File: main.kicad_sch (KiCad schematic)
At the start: 88 parts, among them J1 USB_C_Receptacle, J2 SPIheader, J3 Bus_PCI_Express_x4, J4 chip-annoyers, J5 UART, J6 I2C, U2 SPI_SOIC-8, U3 SPI_DFN-8, Y1 25MHz

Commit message: component arrangement
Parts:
- R1: footprint Resistor_SMD:R_0201_0603Metric -> Resistor_SMD:R_0402_1005Metric
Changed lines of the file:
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@@
 			)
 		)
-		(property "Footprint" "Resistor_SMD:R_0201_0603Metric"
+		(property "Footprint" "Resistor_SMD:R_0402_1005Metric"
 			(at 378.46 132.08 0)
 			(effects

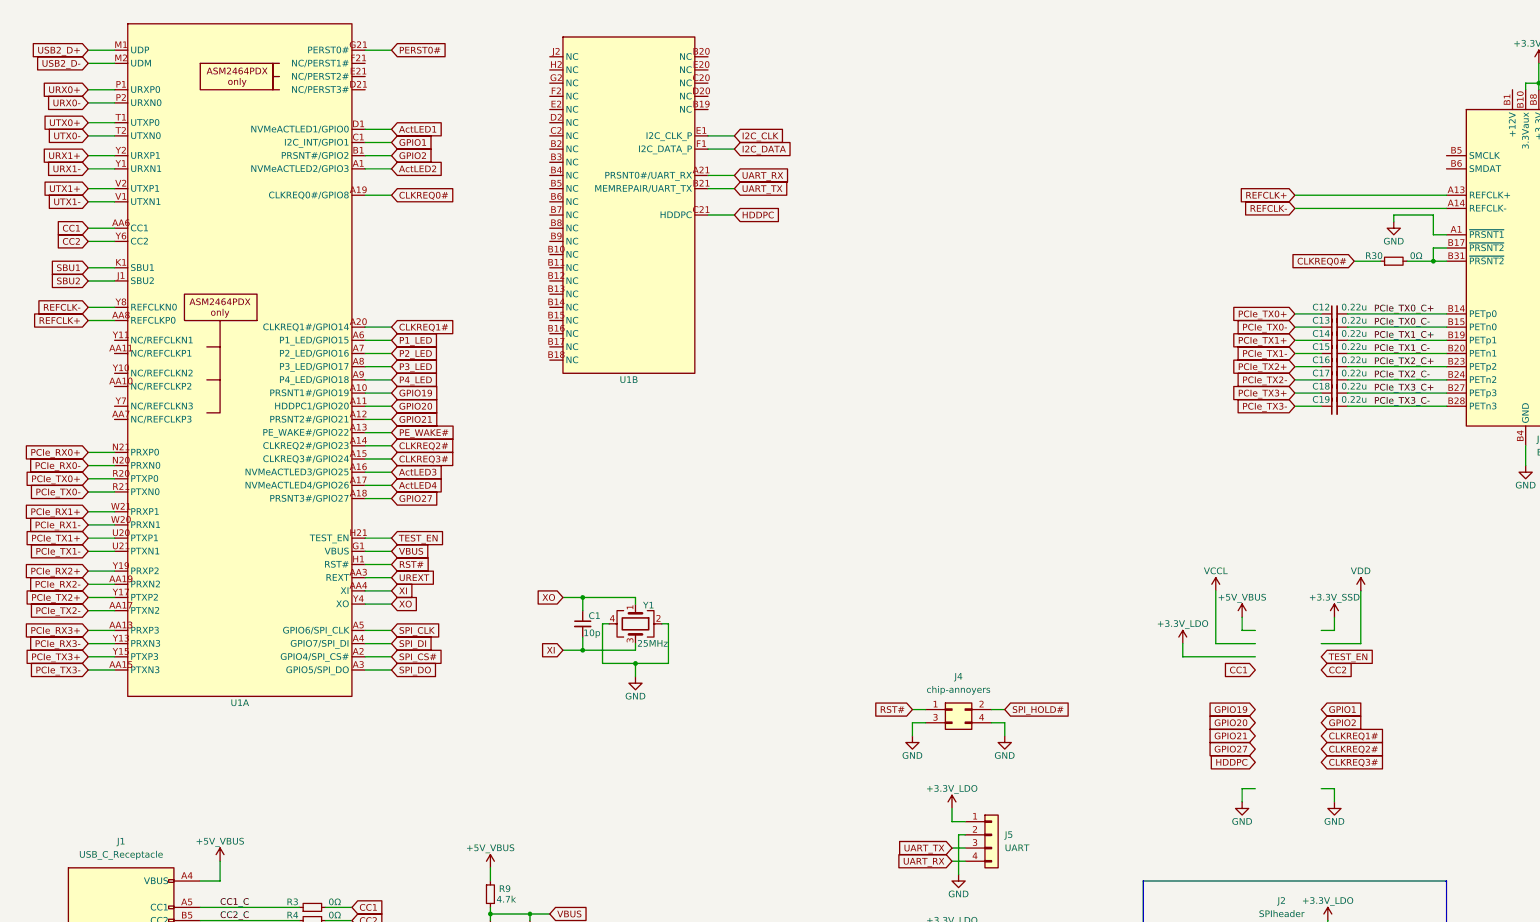
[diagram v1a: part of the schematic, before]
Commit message: A loooot of cool routing and added more connectors
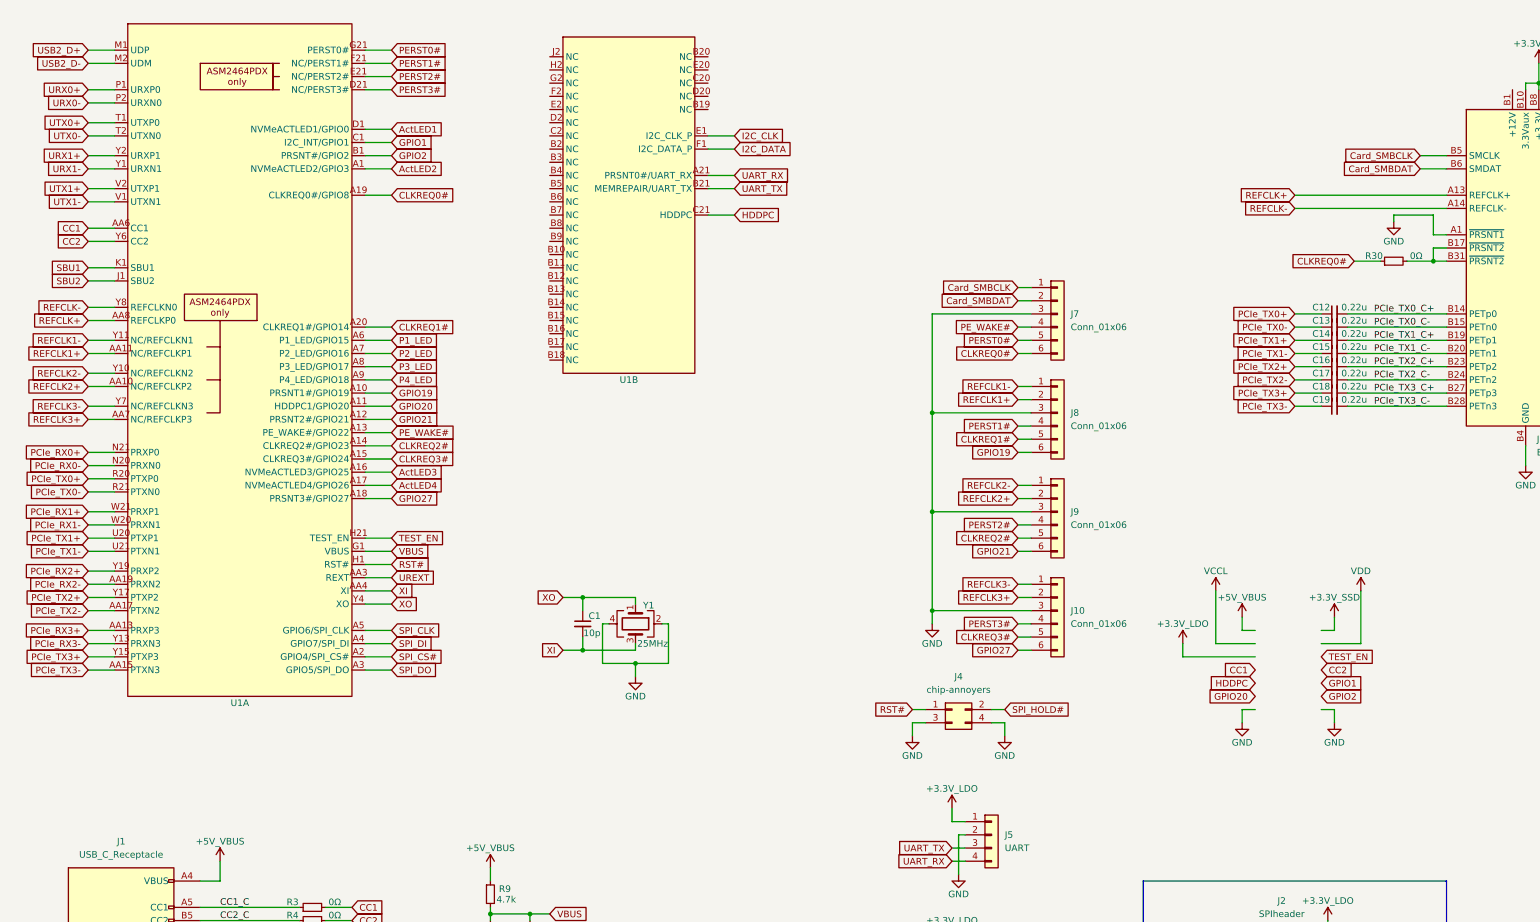
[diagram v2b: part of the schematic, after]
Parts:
- added J10, J7, J8, J9: Conn_01x06, Connector_PinHeader_1.27mm:PinHeader_1x06_P1.27mm_Vertical, symbol Connector_Generic:Conn_01x06
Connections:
- net CLKREQ0#: now also J7.6 (Pin_6)
- net CLKREQ1#: now also J8.5 (Pin_5)
- net CLKREQ2#: now also J9.5 (Pin_5)
- net CLKREQ3#: now also J10.5 (Pin_5)
- net GND: now also J10.3 (Pin_3), J7.3 (Pin_3), J8.3 (Pin_3), J9.3 (Pin_3)
- net GPIO19: now also J8.6 (Pin_6)
- net GPIO21: now also J9.6 (Pin_6)
- net GPIO27: now also J10.6 (Pin_6)
- net PERST0#: now also J7.5 (Pin_5)
- net PE_WAKE#: now also J7.4 (Pin_4)
- net Card_SMBCLK: now reaches J3.B5 (SMCLK)
- net Card_SMBCLK: now also J7.1 (Pin_1)
- net Card_SMBDAT: now reaches J3.B6 (SMDAT)
- net Card_SMBDAT: now also J7.2 (Pin_2)
- net REFCLK2+: now reaches U1.AA10 (NC/REFCLKP2)
- net REFCLK2+: now also J9.2 (Pin_2)
- net REFCLK1+: now reaches U1.AA11 (NC/REFCLKP1)
- net REFCLK1+: now also J8.2 (Pin_2)
- net REFCLK3+: now reaches U1.AA7 (NC/REFCLKP3)
- net REFCLK3+: now also J10.2 (Pin_2)
- net PERST3#: now reaches U1.D21 (NC/PERST3#)
- net PERST3#: now also J10.4 (Pin_4)
- net PERST2#: now reaches U1.E21 (NC/PERST2#)
- net PERST2#: now also J9.4 (Pin_4)
- net PERST1#: now reaches U1.F21 (NC/PERST1#)
- net PERST1#: now also J8.4 (Pin_4)
- net REFCLK2-: now reaches U1.Y10 (NC/REFCLKN2)
- net REFCLK2-: now also J9.1 (Pin_1)
- net REFCLK1-: now reaches U1.Y11 (NC/REFCLKN1)
- net REFCLK1-: now also J8.1 (Pin_1)
- net REFCLK3-: now reaches U1.Y7 (NC/REFCLKN3)
- net REFCLK3-: now also J10.1 (Pin_1)
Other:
- company: (none) -> WifiCable

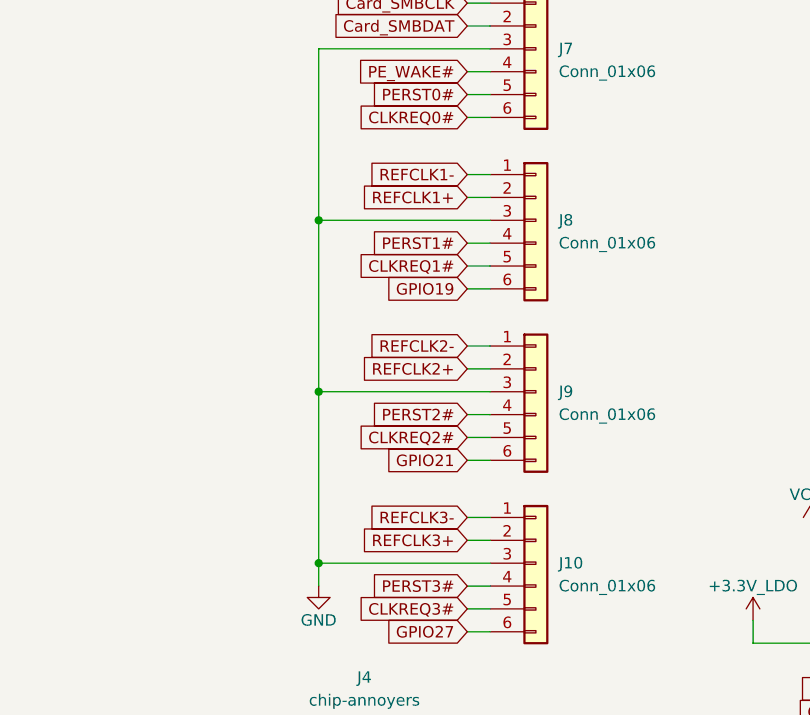
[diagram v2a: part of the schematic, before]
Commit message: Horrible nightmare routing
oh my stars will it do gen 4?
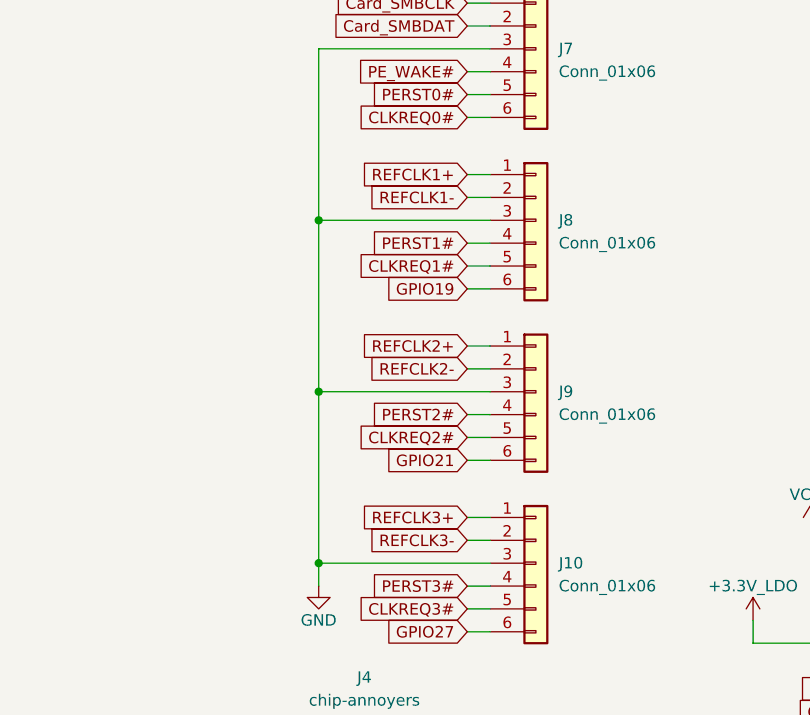
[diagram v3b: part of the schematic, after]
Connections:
- net REFCLK1+: now also J8.1 (Pin_1); no longer J8.2 (Pin_2)
- net REFCLK1-: now also J8.2 (Pin_2); no longer J8.1 (Pin_1)
- net REFCLK2+: now also J9.1 (Pin_1); no longer J9.2 (Pin_2)
- net REFCLK2-: now also J9.2 (Pin_2); no longer J9.1 (Pin_1)
- net REFCLK3+: now also J10.1 (Pin_1); no longer J10.2 (Pin_2)
- net REFCLK3-: now also J10.2 (Pin_2); no longer J10.1 (Pin_1)
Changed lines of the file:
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@@
 	(global_label "REFCLK3-"
 		(shape input)
-		(at 212.09 130.81 180)
+		(at 212.09 133.35 180)
 		(fields_autoplaced yes)
 		(effects
@@
 		)
 		(property "Intersheetrefs" "${INTERSHEET_REFS}"
-			(at 200.4567 130.81 0)
+			(at 200.4567 133.35 0)
 			(effects
 				(font
@@
 	(global_label "REFCLK2-"
 		(shape input)
-		(at 212.09 111.76 180)
+		(at 212.09 114.3 180)
 		(fields_autoplaced yes)
 		(effects
@@
 		)
 		(property "Intersheetrefs" "${INTERSHEET_REFS}"
-			(at 200.4567 111.76 0)
+			(at 200.4567 114.3 0)
 			(effects
 				(font
@@
 	(global_label "REFCLK2+"
 		(shape input)
-		(at 212.09 114.3 180)
+		(at 212.09 111.76 180)
 		(fields_autoplaced yes)
 		(effects
@@
 		)
 		(property "Intersheetrefs" "${INTERSHEET_REFS}"
-			(at 200.4567 114.3 0)
+			(at 200.4567 111.76 0)
 			(effects
 				(font
@@
 	(global_label "REFCLK1+"
 		(shape input)
-		(at 212.09 95.25 180)
+		(at 212.09 92.71 180)
 		(fields_autoplaced yes)
 		(effects
@@
 		)
 		(property "Intersheetrefs" "${INTERSHEET_REFS}"
-			(at 200.4567 95.25 0)
+			(at 200.4567 92.71 0)
 			(effects
 				(font
@@
 	(global_label "REFCLK1-"
 		(shape input)
-		(at 212.09 92.71 180)
+		(at 212.09 95.25 180)
 		(fields_autoplaced yes)
 		(effects
@@
 		)
 		(property "Intersheetrefs" "${INTERSHEET_REFS}"
-			(at 200.4567 92.71 0)
+			(at 200.4567 95.25 0)
 			(effects
 				(font
@@
 	(global_label "REFCLK3+"
 		(shape input)
-		(at 212.09 133.35 180)
+		(at 212.09 130.81 180)
 		(fields_autoplaced yes)
 		(effects
@@
 		)
 		(property "Intersheetrefs" "${INTERSHEET_REFS}"
-			(at 200.4567 133.35 0)
+			(at 200.4567 130.81 0)
 			(effects
 				(font

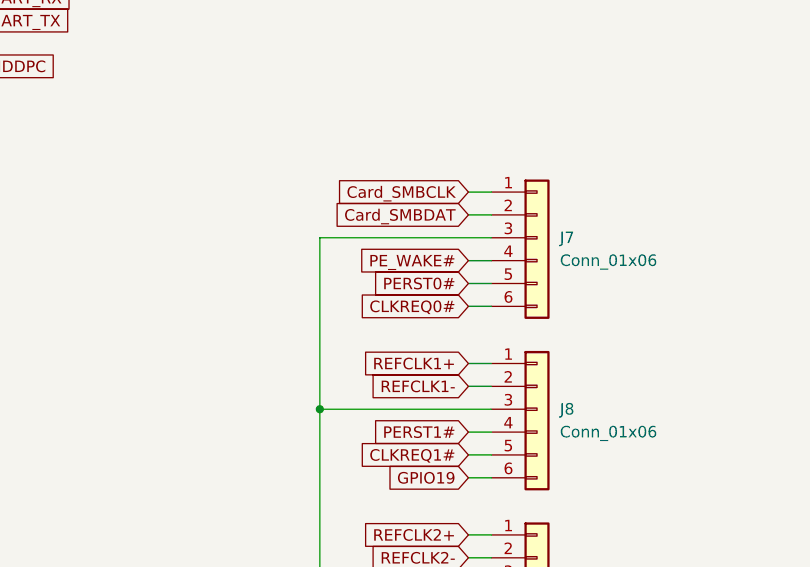
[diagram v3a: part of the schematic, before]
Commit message: some notes
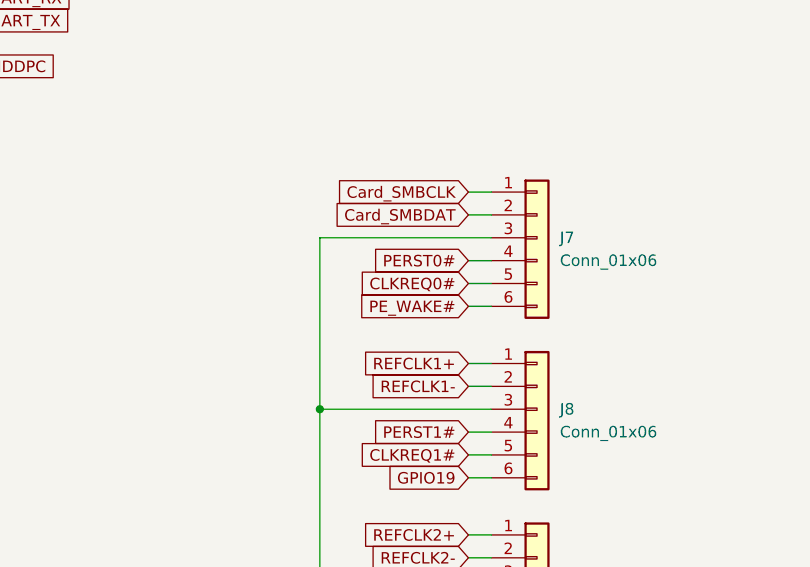
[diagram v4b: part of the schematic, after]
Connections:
- net CLKREQ0#: now also J7.5 (Pin_5); no longer J7.6 (Pin_6)
- net PERST0#: now also J7.4 (Pin_4); no longer J7.5 (Pin_5)
- net PE_WAKE#: now also J7.6 (Pin_6); no longer J7.4 (Pin_4)
